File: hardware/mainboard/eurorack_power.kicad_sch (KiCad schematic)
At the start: 11 parts, among them J1 Eurorack PWR

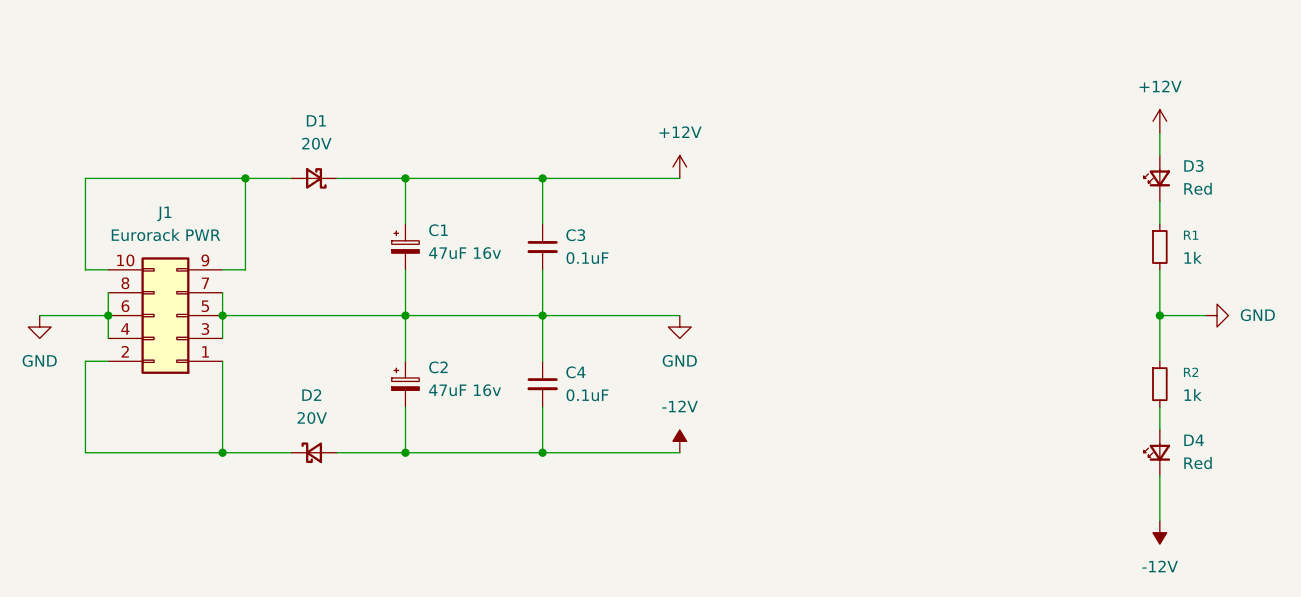
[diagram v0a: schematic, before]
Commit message: Layout
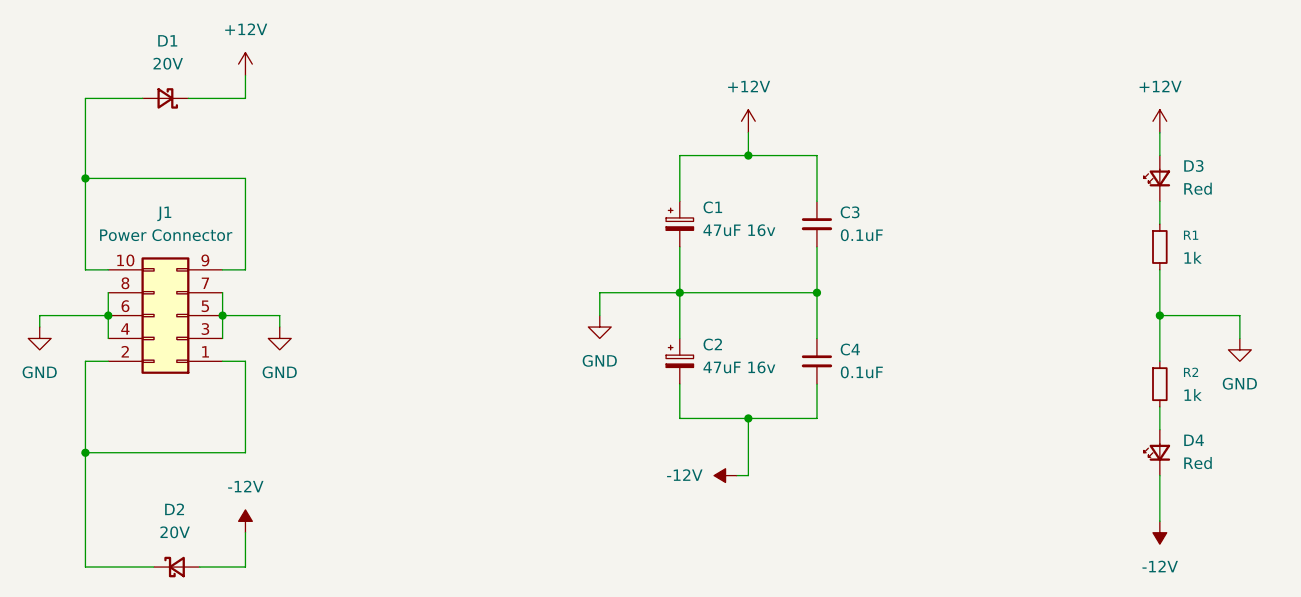
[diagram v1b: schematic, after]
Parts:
- J1: value Eurorack PWR -> Power Connector; footprint Connector_IDC:IDC-Header_2x05_P2.54mm_Latch6.5mm_Vertical -> Connector_IDC:IDC-Header_2x05_P2.54mm_Vertical
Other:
- moved on the sheet: C1, C2, C3, C4, D2

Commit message: Sent mainboard
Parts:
- C1, C2: LCSC_Part_No (none) -> C311666; Manufacturer (none) -> Lelon; Manufacturer_Part_No (none) -> OVK470M1ETR-0606
- C3, C4: LCSC_Part_No (none) -> C49678; Manufacturer (none) -> YAGEO; Manufacturer_Part_No (none) -> CC0805KRX7R9BB104
- D1, D2: LCSC_Part_No (none) -> C114696; Manufacturer (none) -> Nexperia; Manufacturer_Part_No (none) -> BAT46WJ,115
- D3, D4: LCSC_Part_No (none) -> C19171391; Manufacturer (none) -> YONGYUTAI; Manufacturer_Part_No (none) -> YLED0805R
- J1: LCSC_Part_No (none) -> C573025; Manufacturer (none) -> TE Connectivity; Manufacturer_Part_No (none) -> 1761681-3
- R1, R2: LCSC_Part_No (none) -> C17513; Manufacturer (none) -> UNI-ROYAL; Manufacturer_Part_No (none) -> 0805W8F1001T5E
